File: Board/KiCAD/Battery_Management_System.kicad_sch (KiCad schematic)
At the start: 19 parts, among them J1 Conn_01x06_Socket, J10 Conn_01x02, J11 Conn_01x02, J12 Conn_01x02, J13 Conn_01x02, J5 Conn_01x03, J7 Conn_01x05, J8 Conn_01x02, J9 Conn_01x02

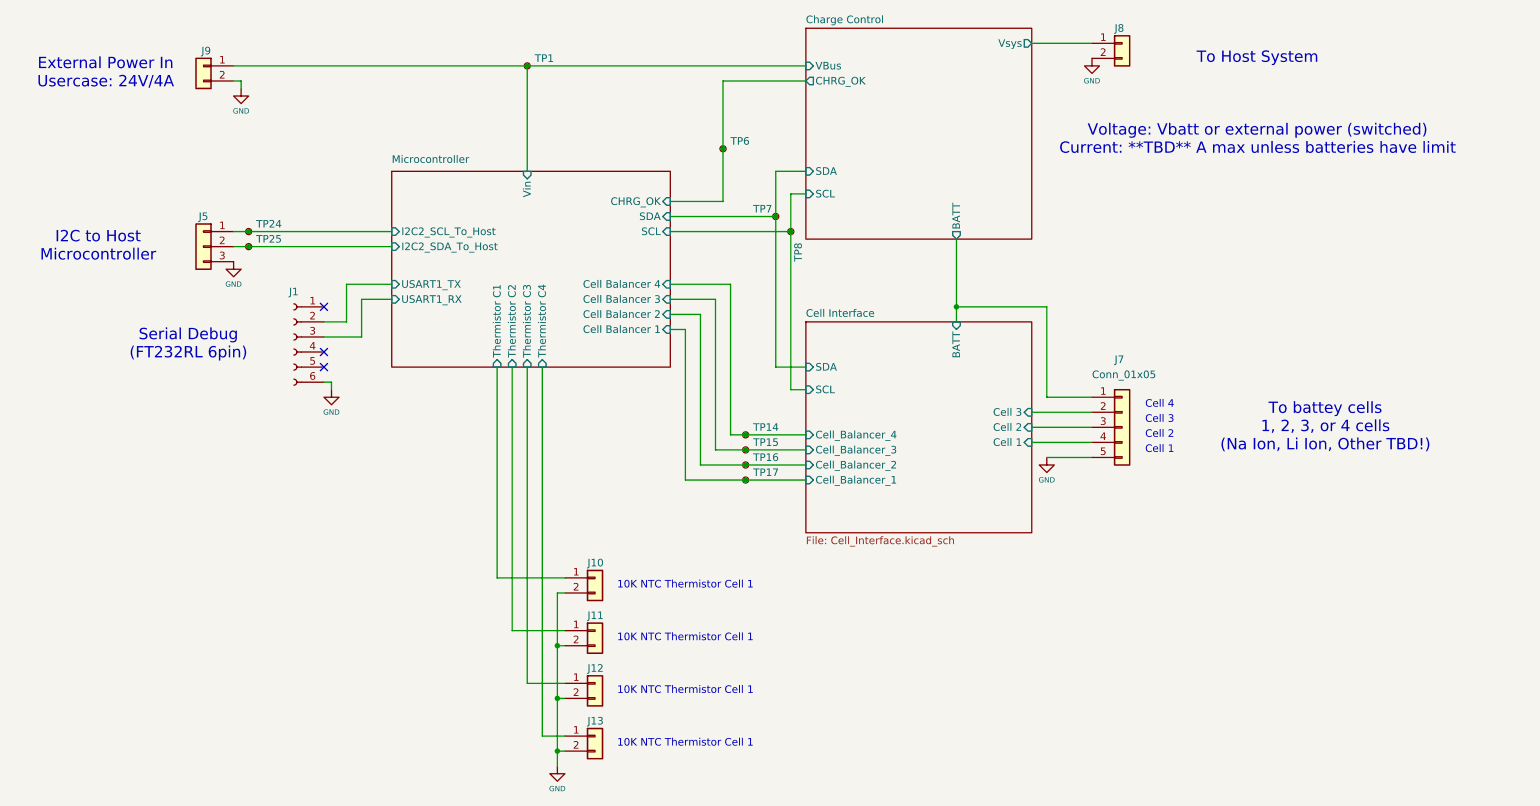
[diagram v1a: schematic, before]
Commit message: BOM Complete Need a Once Over Check
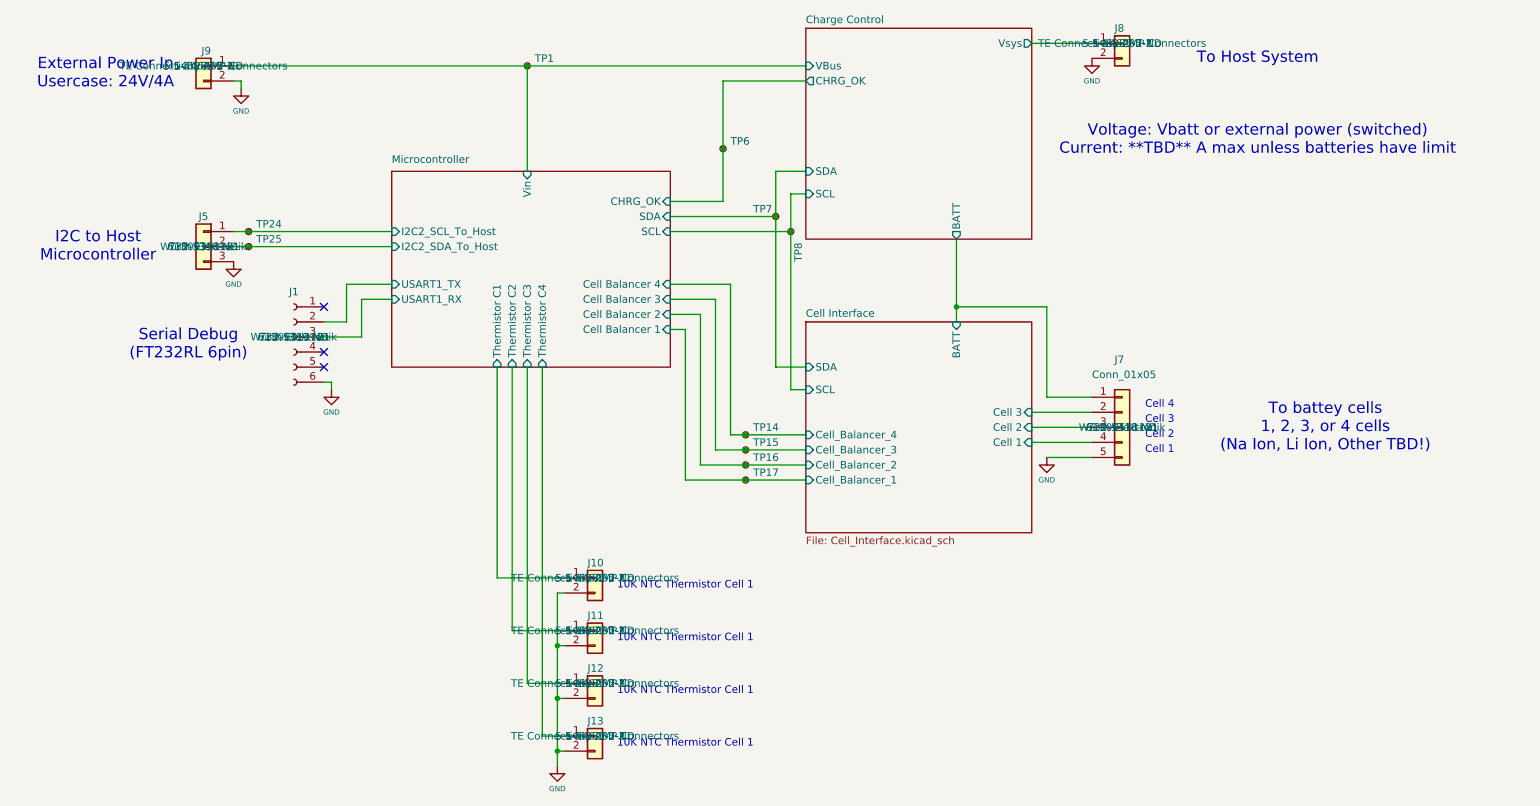
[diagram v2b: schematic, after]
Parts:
- J1: MFR (none) -> Würth Elektronik; MPN (none) -> 732-5319-ND; Package (none) -> 61300611121
- J10, J11, J12, J13, J8, J9: MFR (none) -> TE Connectivity AMP Connectors; MPN (none) -> 5-146285-2-ND; Package (none) -> 5-146285-2
- J5: MFR (none) -> Würth Elektronik; MPN (none) -> 732-5316-ND; Package (none) -> 61300311121
- J7: MFR (none) -> Würth Elektronik; MPN (none) -> 732-5318-ND; Package (none) -> 61300511121
